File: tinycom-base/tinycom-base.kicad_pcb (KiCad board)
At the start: 2 copper layers, 45.2 x 45.2 mm, 38 parts, among them J1 MICRO_SD_HINGE, P1 CONN_02X08, P2 CONN_02X08, P3 USB_A, P4 USB_OTG, U1 SY8008BAAC, U2 SY8008BAAC, U3 SY8008BAAC

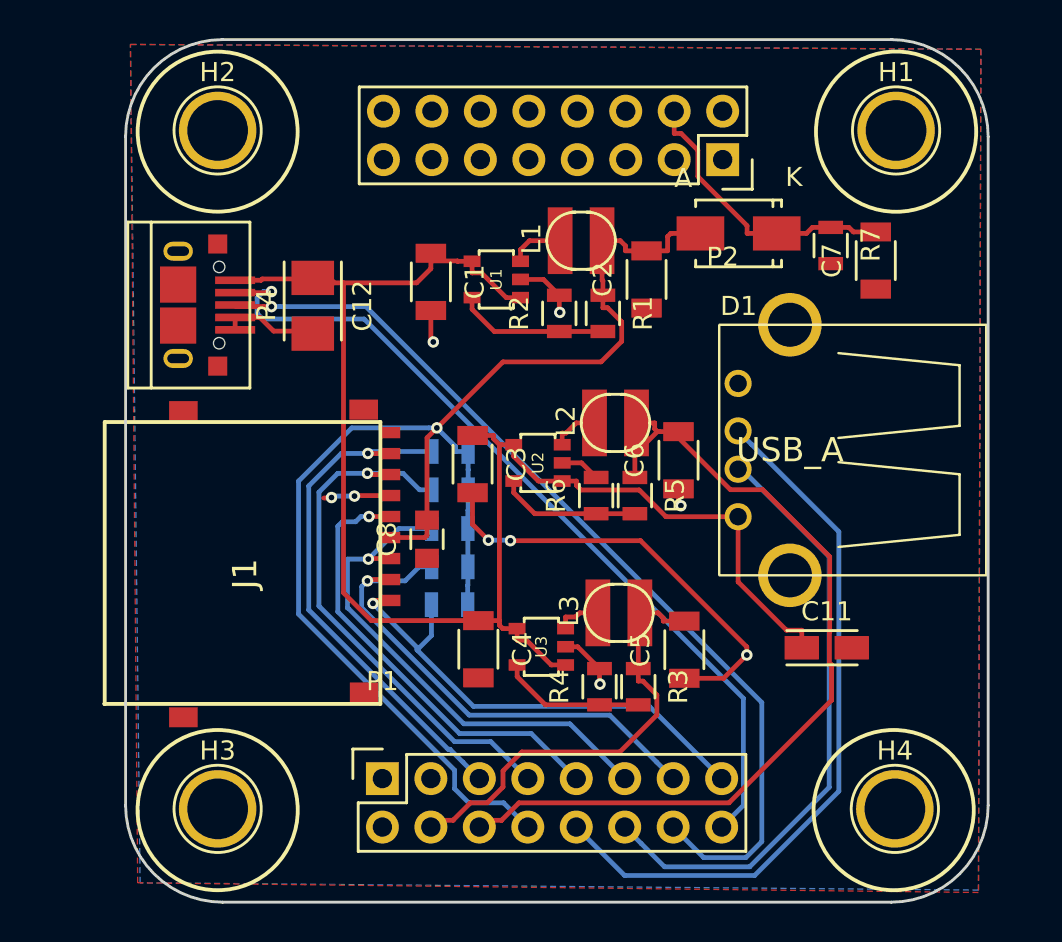
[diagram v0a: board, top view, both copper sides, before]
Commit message: rename wifi->basse
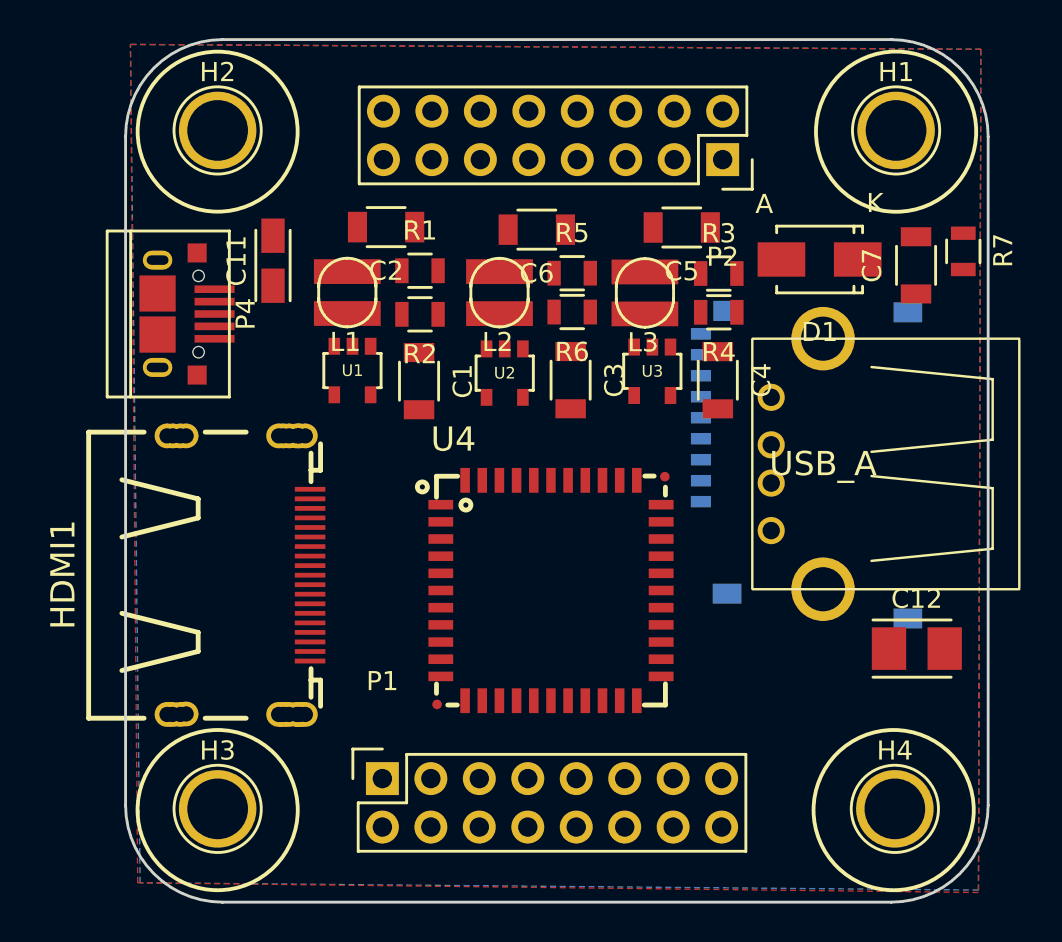
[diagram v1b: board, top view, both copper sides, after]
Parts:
- removed C8: C_Small, Capacitors_SMD:C_0805
- removed R10, R11, R12, R8, R9: R_Small, Resistors_SMD:R_0805
- added HDMI1: HDMI-SWM-19, tinycom:HDMI-SWM-19, F.Cu at (128.6, 107.3)
- added U4: RTL8723BS(ComboModule), tinycom:RL-SM02BD(RTL8723BS), F.Cu at (146.8, 108.1)
- J1: moved to B.Cu
- moved J1 44.2 mm to (168.4, 102.1)
- moved C12 36.4 mm to (165.9, 111.2), turned to 0 degrees
- moved C11 35.4 mm to (132.2, 90.8), turned to 90 degrees
- moved C5 22.1 mm to (153.6, 89.1), turned to 180 degrees
- moved R3 22.1 mm to (155.6, 91.5), turned to 0 degrees
- moved R4 20.6 mm to (155.6, 93.5), turned to 180 degrees
- moved C4 18.9 mm to (155.5, 97.1)
- moved L3 16.8 mm to (151.7, 92.5), turned to 180 degrees
- moved U3 15.6 mm to (152.1, 96.6), turned to 180 degrees
- moved C6 14.2 mm to (146.0, 89.2), turned to 180 degrees
- moved C2 13.9 mm to (138.1, 89.1), turned to 180 degrees
- moved L1 12.6 mm to (136.1, 92.5), turned to 180 degrees
- moved R5 12.1 mm to (147.9, 91.5), turned to 0 degrees
- moved R1 9.84 mm to (139.9, 91.4), turned to 0 degrees
- moved R6 9.70 mm to (147.9, 93.5), turned to 180 degrees
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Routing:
- net +5V: track 81.5 -> 0.00 mm
- net VCC_33: track 74.5 -> 0.00 mm, vias 1 -> 0
- net UDP0: track 49.2 -> 0.00 mm, vias 1 -> 0
- net VCC_14: track 45.3 -> 0.00 mm
- net UDM0: track 44.7 -> 0.00 mm, vias 1 -> 0
- net GND: track 42.7 -> 0.00 mm, vias 9 -> 0
- net UDP1: track 37.7 -> 0.00 mm
- net UDM1: track 32.6 -> 0.00 mm
- net SDC0_D0: track 28.6 -> 0.00 mm, vias 1 -> 0
- net SDC0_D1: track 27.5 -> 0.00 mm, vias 1 -> 0
- net SDC0_CMD: track 27.0 -> 0.00 mm, vias 1 -> 0
- net SDC0_D3: track 26.5 -> 0.00 mm, vias 1 -> 0
- net SDC0_D2: track 25.8 -> 0.00 mm, vias 1 -> 0
- net SDC0_CLK: track 23.6 -> 0.00 mm, vias 1 -> 0
- net VCC_15: track 23.4 -> 0.00 mm
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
